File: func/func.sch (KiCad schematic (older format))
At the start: 36 parts, among them SW1 SW_MEC_5G, SW2 SW_MEC_5G, SW3 SW_MEC_5G, SW4 SW_MEC_5G, SW5 SW_MEC_5G

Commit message: Replaced fung
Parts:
- removed U?: CA56-12CGKWA, Display_7Segment:CA56-12CGKWA, symbol Display_Character:CA56-12CGKWA
- added U?: CA56-12CGKWA, Display_7Segment:CA56-12CGKWA, symbol FUNG:CA56-12CGKWA
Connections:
- net labels removed: CS, DIO, GRID1, GRID2, GRID3, GRID4, GRID5, GRID6, K1, K2, MISO, MOSI, PA0, PA1, PA2, PA3, PA4, PA5, PA6, PA7, PB0, PB1, PB2, PB3, PB4, PB5, PB6, PB7, PC0, PC1, PC2, PC3, PC4, PC5, PC6, PC7, PD0, PD1, PD2, PD3, PD4, PD5, PD6, PD7, PE0, PE1, PE2, SCK, ~CE, ~OE, ~SS, ~WE
- wire segments 106 -> 102
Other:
- note added: "к ПЭВМ"
- note removed: "CLK"
- note removed: "К ПЭВМ"

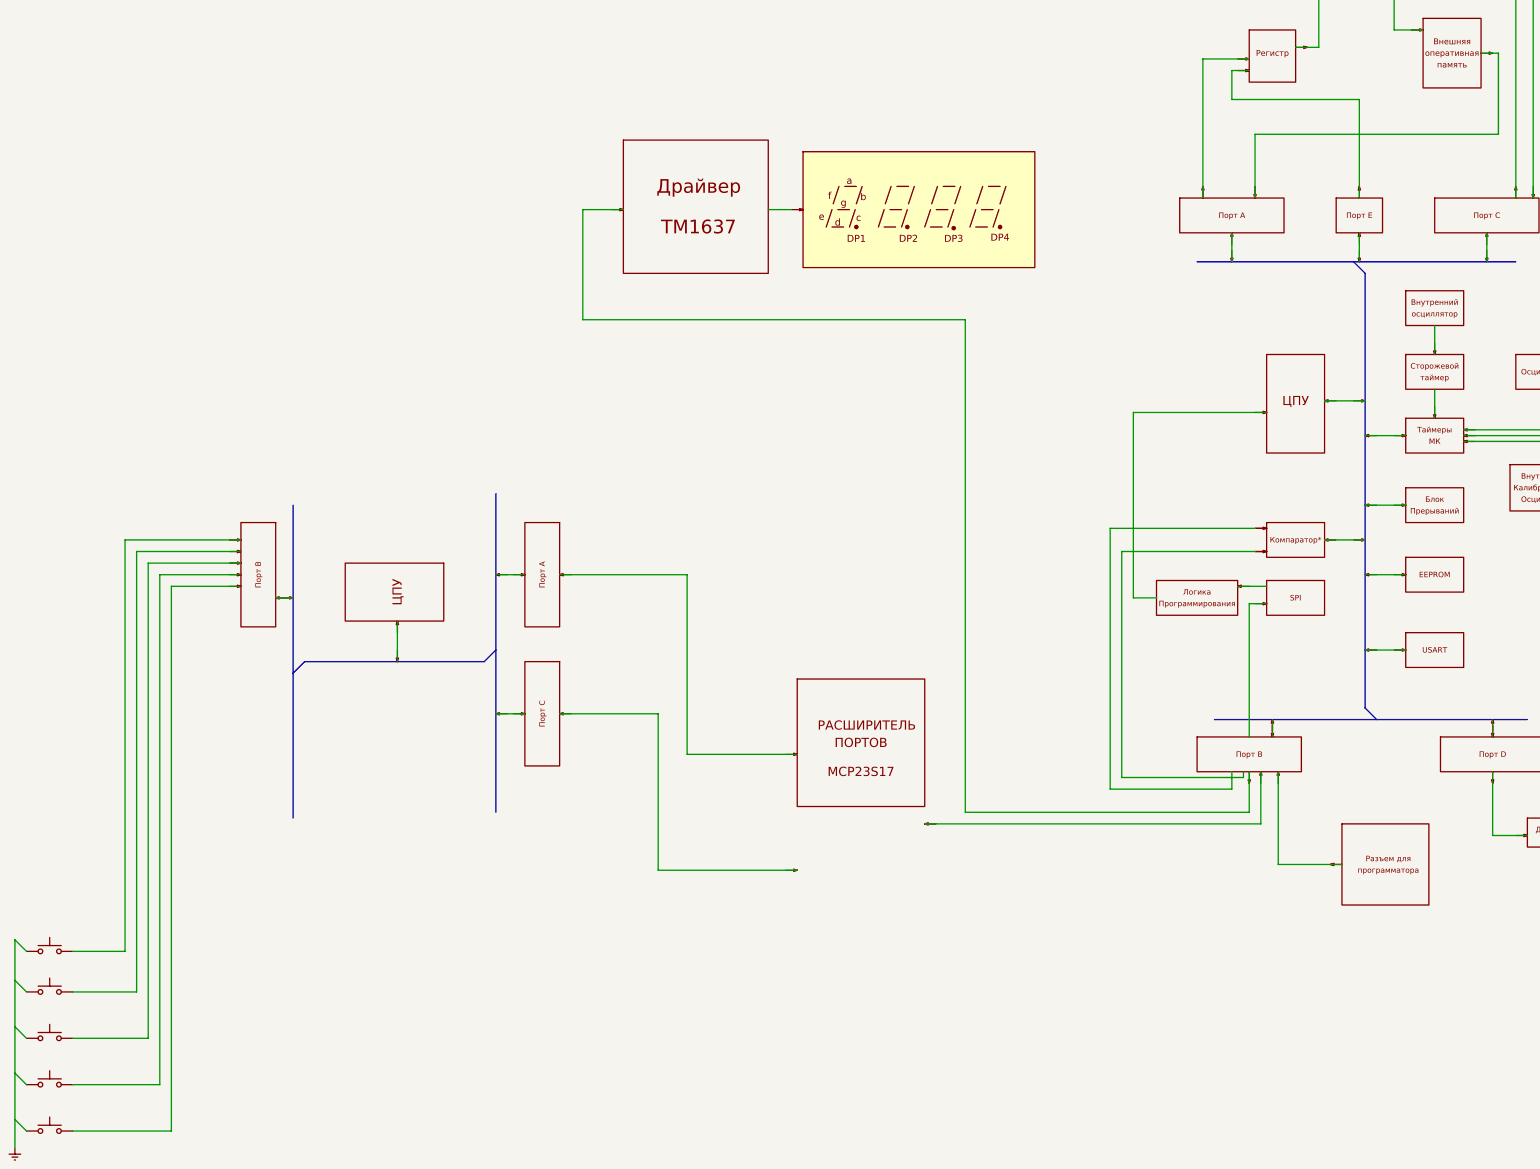
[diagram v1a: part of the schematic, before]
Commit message: Almost ready
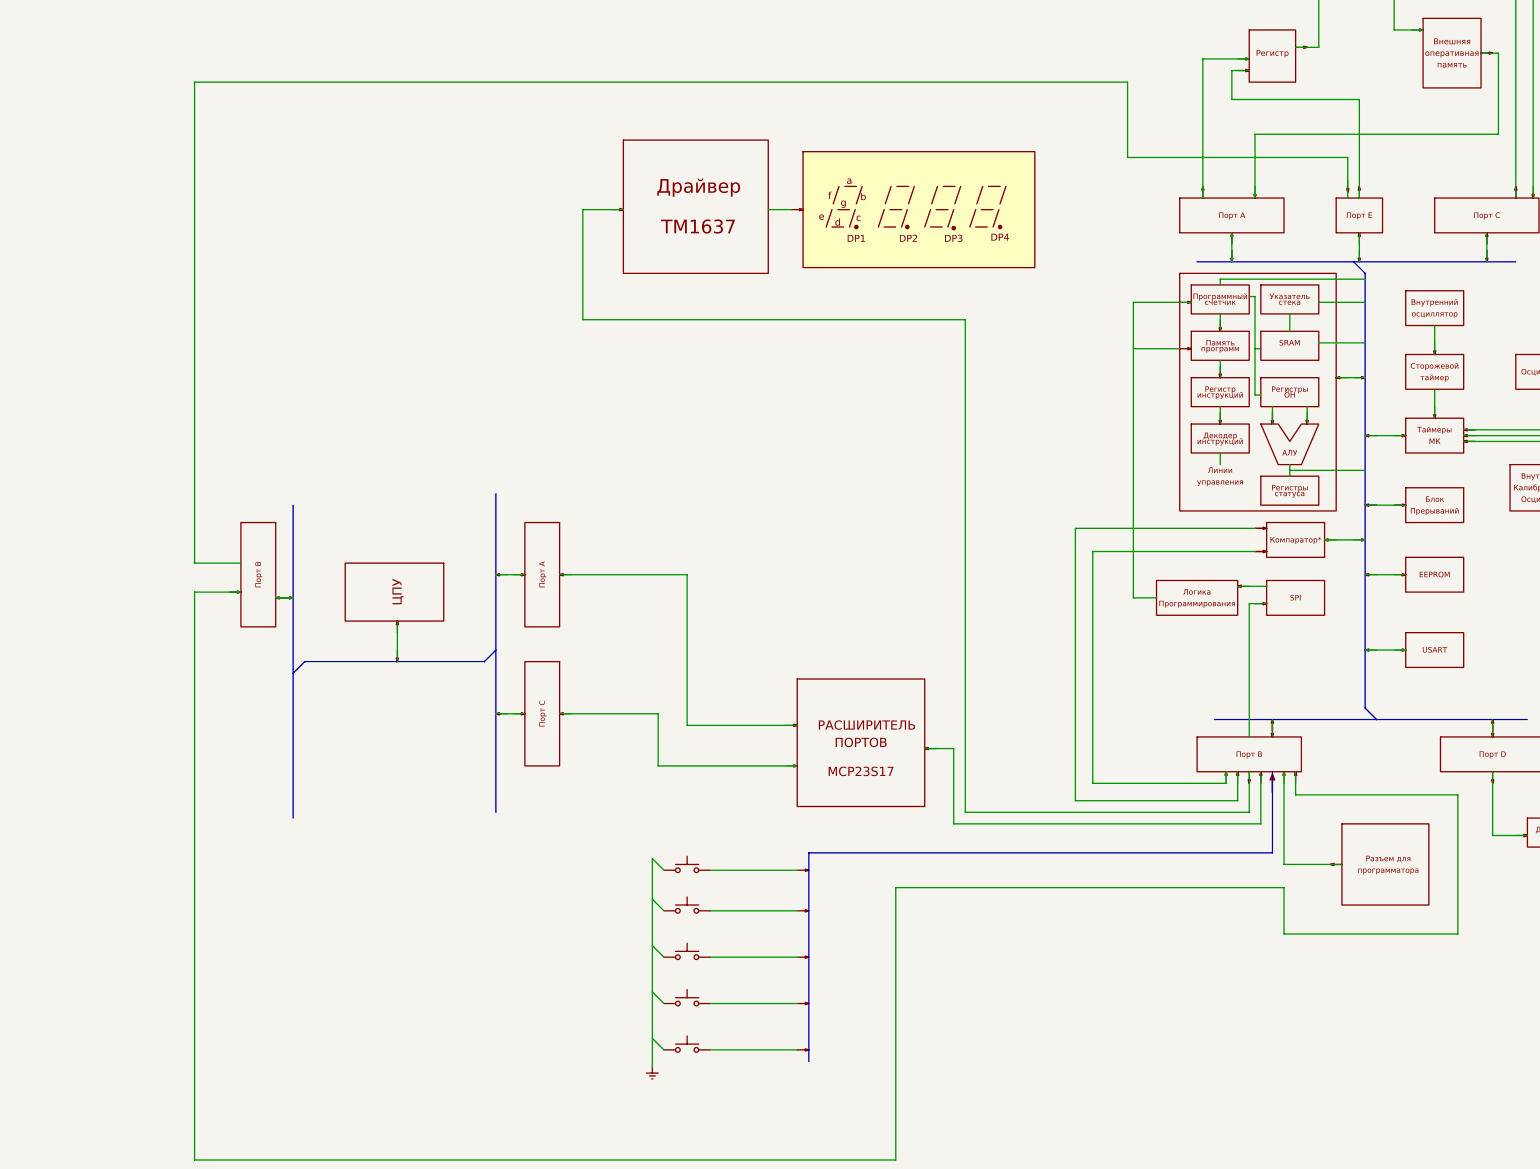
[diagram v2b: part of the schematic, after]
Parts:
- removed SW1: SW_MEC_5G, symbol Switch:SW_MEC_5G
- removed U?: CPU, symbol FUNG:CPU
- added SW?: SW_MEC_5G, symbol Switch:SW_MEC_5G
- added U?: CPU_copy, symbol FUNG:CPU_copy
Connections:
- wire segments 102 -> 128

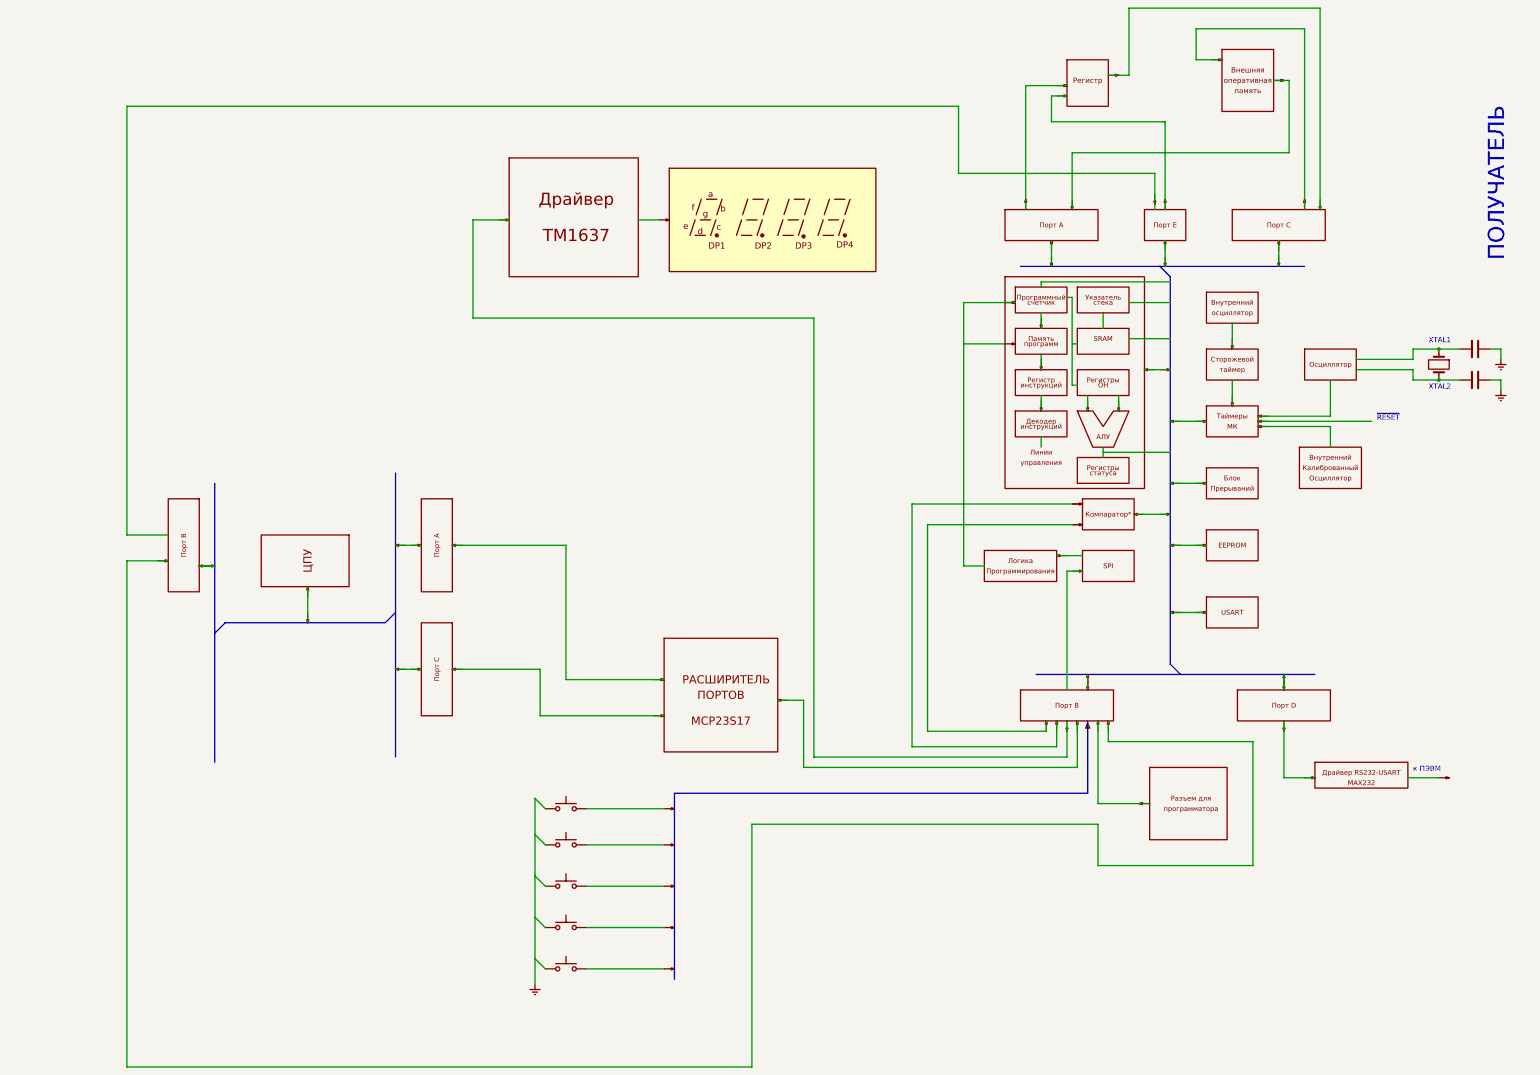
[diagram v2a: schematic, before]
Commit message: update prinsip
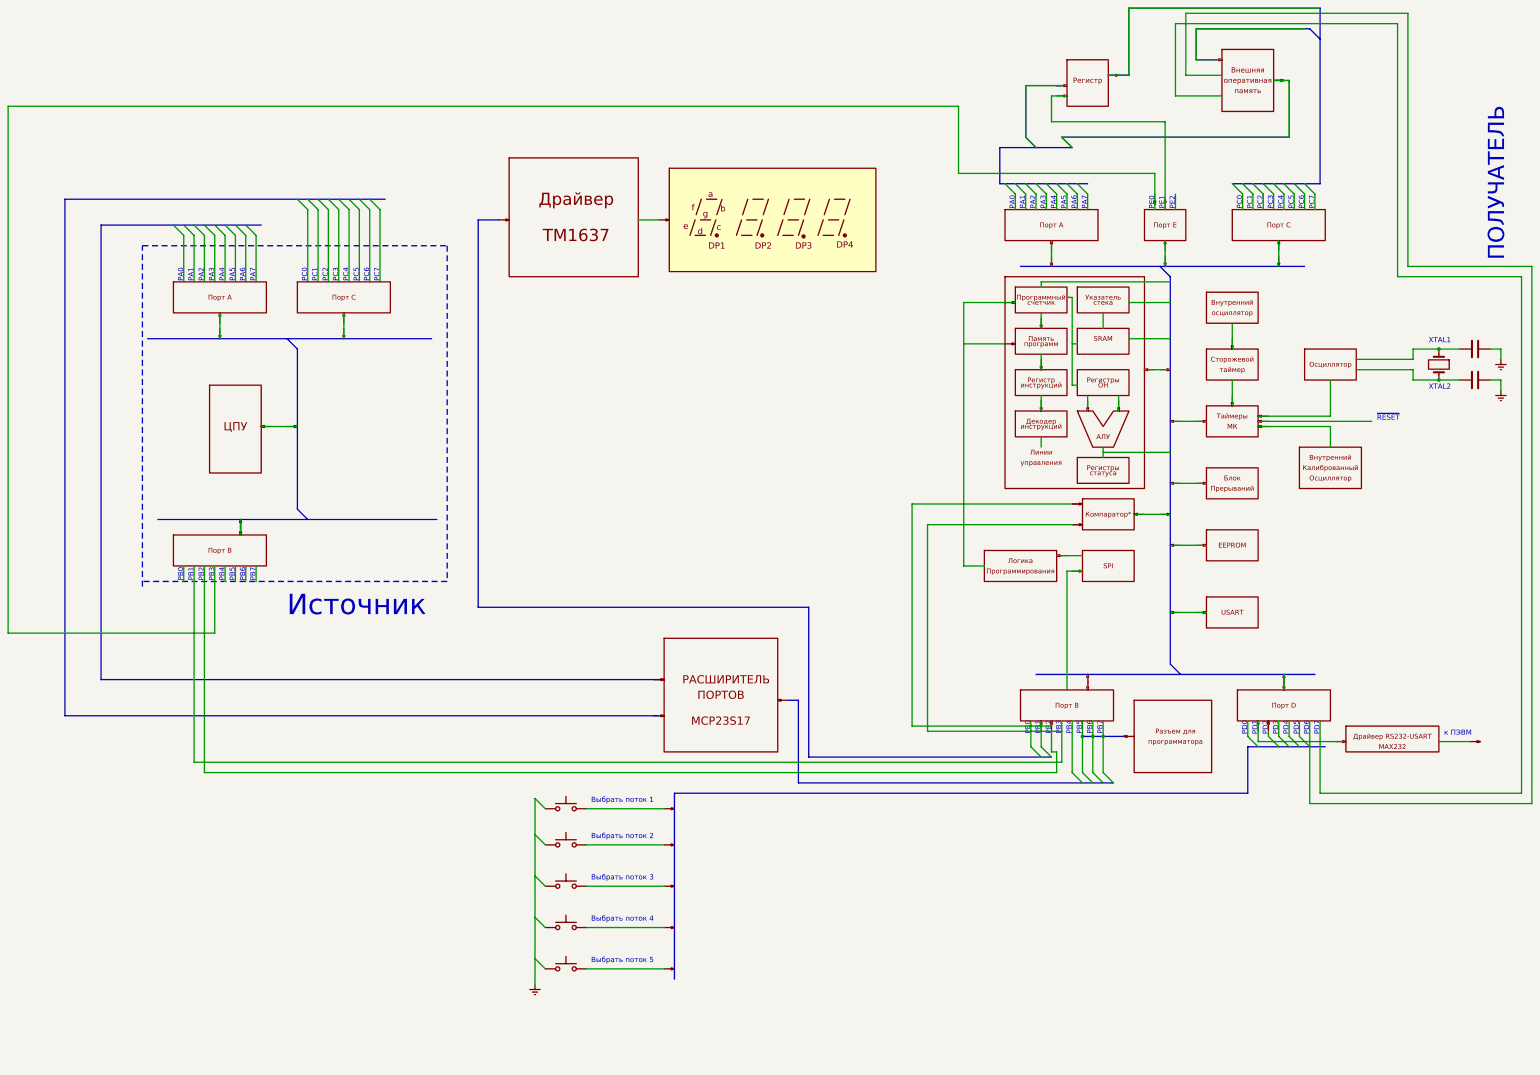
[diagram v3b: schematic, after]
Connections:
- wire segments 128 -> 173
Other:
- note added: "PA0"
- note added: "PA1"
- note added: "PA2"
- note added: "PA3"
- note added: "PA4"
- note added: "PA5"
- note added: "PA6"
- note added: "PA7"
- note added: "PB0"
- note added: "PB1"
- note added: "PB2"
- note added: "PB3"
- note added: "PB4"
- note added: "PB5"
- note added: "PB6"
- note added: "PB7"
- note added: "PC0"
- note added: "PC1"
- note added: "PC2"
- note added: "PC2\n"
- note added: "PC3"
- note added: "PC4"
- note added: "PC5"
- note added: "PC6"
- note added: "PC7"
- note added: "PD0"
- note added: "PD1"
- note added: "PD2"
- note added: "PD3"
- note added: "PD4"
- note added: "PD5"
- note added: "PD6"
- note added: "PD7"
- note added: "PE0"
- note added: "PE1"
- note added: "PE2"
- note added: "Выбрать поток 1"
- note added: "Выбрать поток 2"
- note added: "Выбрать поток 3"
- note added: "Выбрать поток 4"
- note added: "Выбрать поток 5"
- note added: "Источник"
